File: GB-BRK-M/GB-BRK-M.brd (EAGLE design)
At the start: 49.3 x 48 mm, 2 parts

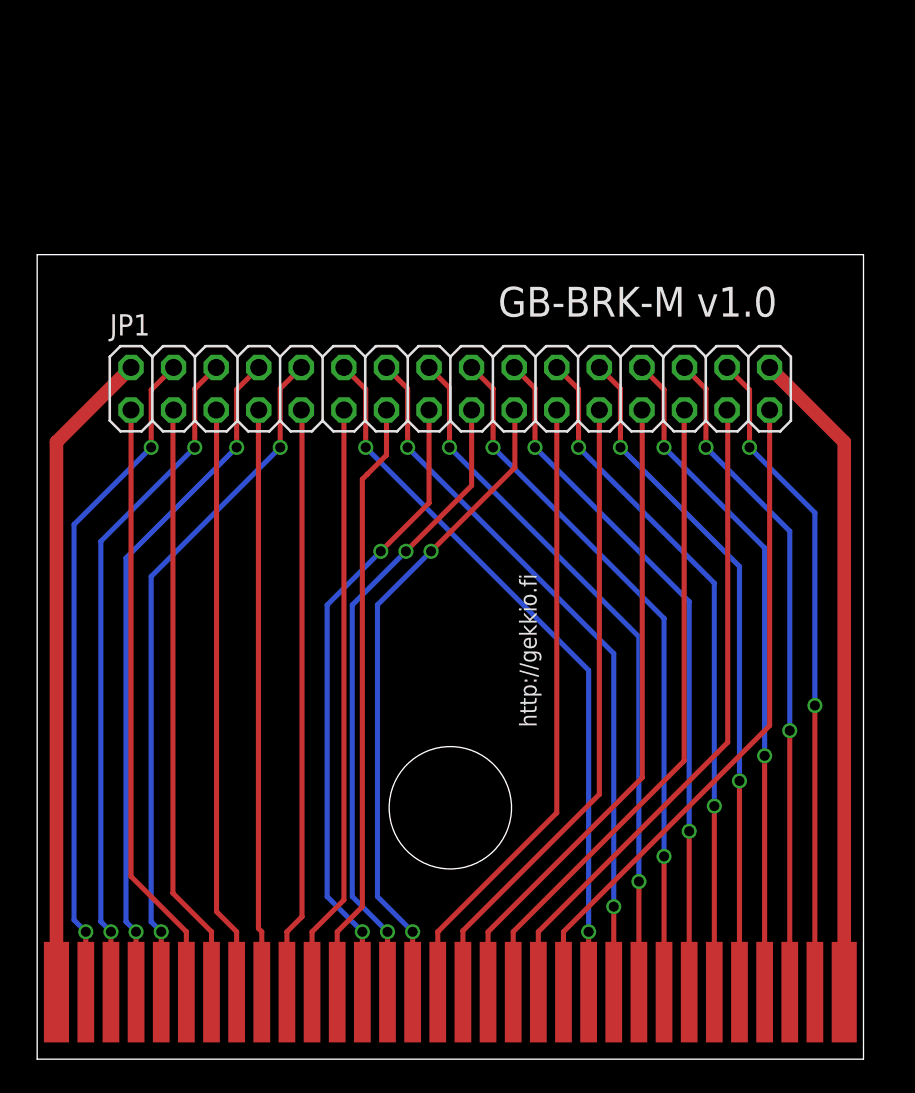
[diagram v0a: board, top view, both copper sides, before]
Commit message: GB-BRK-M v2.1
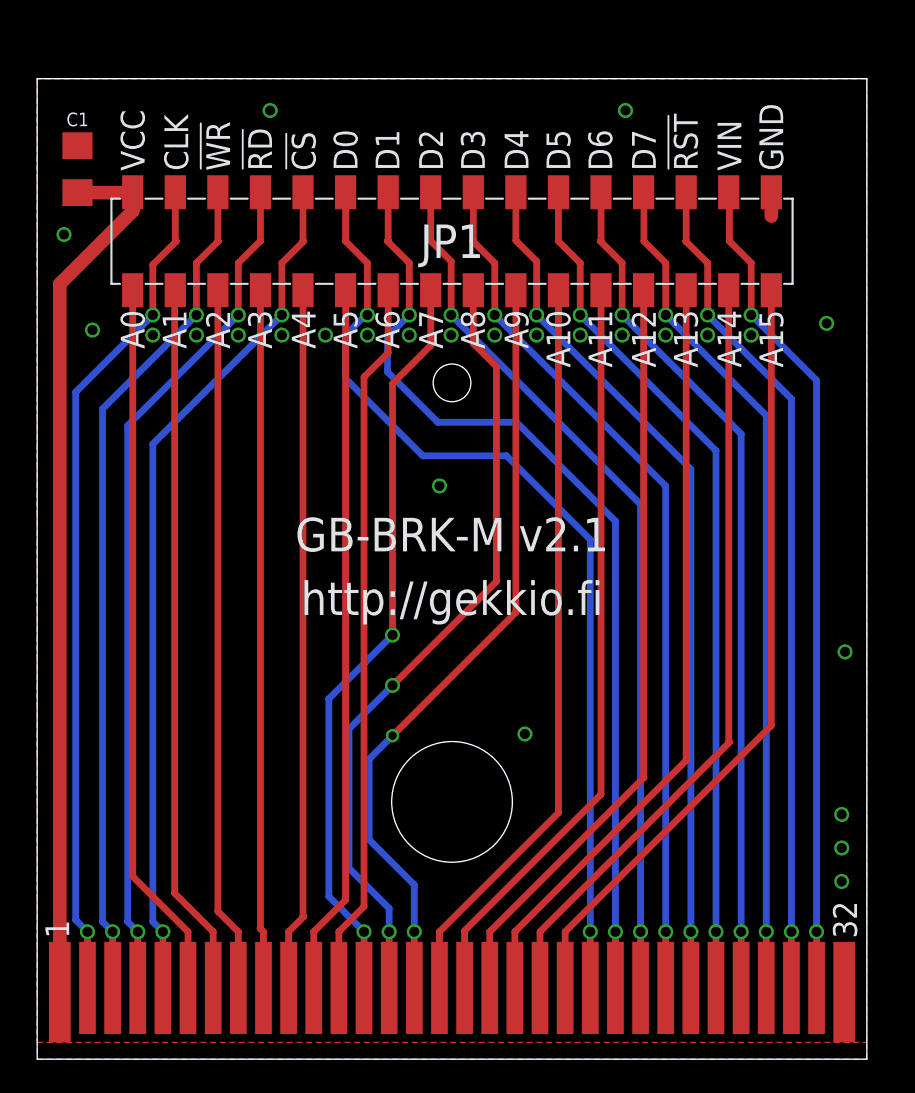
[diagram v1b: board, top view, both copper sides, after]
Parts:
- added C1: 0.1uF, SparkFun-Capacitors:1206
- JP1: device pinhead:2X16 -> pinhead+:2X16_SMT
- moved JP1 8.80 mm to (24.8, 48.8)
- moved U$2 0.10 mm to (24.0, 4.00)
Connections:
- net MREQ renamed !CS
- net RD renamed !RD
- net RST renamed !RST
- net WR renamed !WR
- net GND: now also C1.2
- net VCC: now also C1.1
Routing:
- net GND: track 39.1 -> 1.42 mm, vias 0 -> 26
- net D0: track 43.3 -> 57.6 mm
- net D1: track 42.9 -> 57.0 mm
- net VCC: track 39.3 -> 52.8 mm
- net CLK: track 40.0 -> 50.3 mm
- net !CS: track 41.2 -> 51.5 mm
- net !WR: track 40.4 -> 50.6 mm
- net !RST: track 39.9 -> 50.1 mm
- net D7: track 40.3 -> 50.5 mm
- net !RD: track 40.8 -> 51.0 mm
- net VIN: track 39.5 -> 49.6 mm
- net D2: track 42.5 -> 52.7 mm
- net D6: track 40.8 -> 51.0 mm
- net D3: track 42.1 -> 52.2 mm
- net D5: track 41.3 -> 51.4 mm
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- added copper zone on layer 1, net GND
- added copper zone on layer 16, net GND
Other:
- board size 49.3 x 48 mm -> 49.5 x 58.5 mm
- board text added: "!CS"
- board text added: "!RD"
- board text added: "!RST"
- board text added: "!WR"
- board text added: "1"
- board text added: "32"
- board text added: "A0"
- board text added: "A1"
- board text added: "A10"
- board text added: "A11"
- board text added: "A12"
- board text added: "A13"
- board text added: "A14"
- board text added: "A15"
- board text added: "A2"
- board text added: "A3"
- board text added: "A4"
- board text added: "A5"
- board text added: "A6"
- board text added: "A7"
- board text added: "A8"
- board text added: "A9"
- board text added: "CLK"
- board text added: "D0"
- board text added: "D1"
- board text added: "D2"
- board text added: "D3"
- board text added: "D4"
- board text added: "D5"
- board text added: "D6"
- board text added: "D7"
- board text added: "GB-BRK-M v2.1"
- board text added: "GND"
- board text added: "VCC"
- board text added: "VIN"
- board text removed: "GB-BRK-M v1.0"
